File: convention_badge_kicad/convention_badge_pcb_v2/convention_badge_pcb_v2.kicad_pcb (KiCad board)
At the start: 4 copper layers, 90 x 98 mm, 56 parts, among them J1 USBC, J2 Conn_01x03_Pin, J3 3.7V Battery, J4 Conn_01x07_Pin, J5 Conn_01x07_Pin, Q1 AO3401A, SW1 SW4X2, SW2 SW4X2, SW3 SW_Push, SW4 SW_Push, SW5 SW_Push, SW6 SW4X2, U1 ESP32-C3-WROOM-02, U2 FS8205A, U3 TP4056, U4 DW01A, U5 TLV75733PDBV

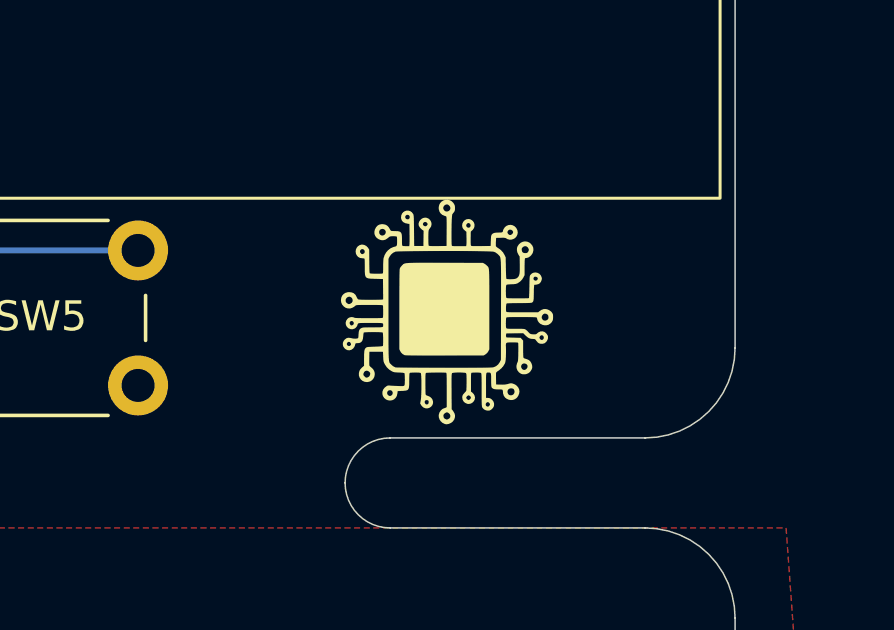
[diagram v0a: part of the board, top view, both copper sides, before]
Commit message: submitted to jlcpcb
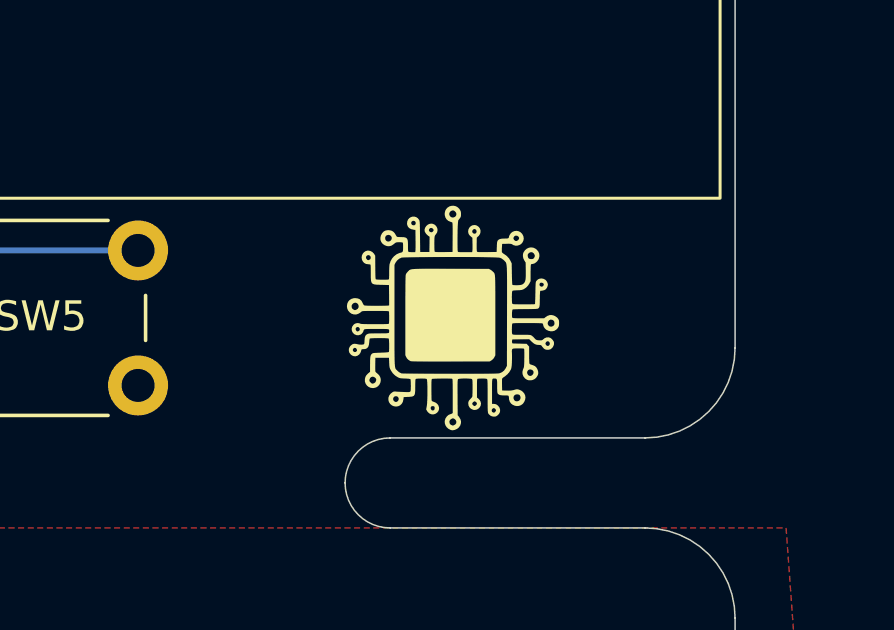
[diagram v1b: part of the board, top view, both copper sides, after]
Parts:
- moved G*** 0.28 mm to (190.2, 123.0)
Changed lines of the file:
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@@
 		(allow_soldermask_bridges_in_footprints no)
 		(tenting front back)
+		(aux_axis_origin 109.6 149)
+		(grid_origin 109.6 149)
 		(pcbplotparams
 			(layerselection 0x00000000_00000000_55555555_575555ff)
@@
 	(footprint "LOGO"
 		(layer "F.Cu")
-		(at 190 122.8)
+		(at 190.2 123)
 		(property "Reference" "G***"
 			(at 0 0 0)
@@
 			)
 		)
+		(property "LCSC" "C2337"
+			(at 0 0 0)
+			(unlocked yes)
+			(layer "F.Fab")
+			(hide yes)
+			(effects
+				(font
+					(size 1 1)
+					(thickness 0.15)
+				)
+			)
+		)
 		(property ki_fp_filters "Connector*:*_1x??_*")
 		(sheetname "/")
@@
 			)
 		)
+		(property "LCSC" ""
+			(at 0 0 0)
+			(unlocked yes)
+			(layer "F.Fab")
+			(hide yes)
+			(effects
+				(font
+					(size 1 1)
+					(thickness 0.15)
+				)
+			)
+		)
 		(property ki_fp_filters "Connector*:*_1x??_*")
 		(sheetname "/")
@@
 			)
 		)
+		(property "LCSC" ""
+			(at 0 0 270)
+			(unlocked yes)
+			(layer "F.Fab")
+			(hide yes)
+			(effects
+				(font
+					(size 1 1)
+					(thickness 0.15)
+				)
+			)
+		)
 		(property ki_fp_filters "Connector*:*_1x??_*")
 		(sheetname "/")
@@
 			)
 		)
-		(property "LCSC" " C318884"
+		(property "LCSC" "C318884"
 			(at 0 0 0)
 			(unlocked yes)
@@
 			)
 		)
-		(property "LCSC" "C1590"
+		(property "LCSC" "C14663"
 			(at 0 0 0)
 			(unlocked yes)
@@
 			)
 		)
-		(property "LCSC" " C485517"
+		(property "LCSC" "C485517"
 			(at 0 0 180)
 			(unlocked yes)
@@
 			)
 		)
-		(property "LCSC" "C1590"
+		(property "LCSC" "C14663"
 			(at 0 0 270)
 			(unlocked yes)
@@
 			)
 		)
-		(property "LCSC" "C2287"
+		(property "LCSC" "C2290"
 			(at 0 0 0)
 			(unlocked yes)
@@
 			)
 		)
-		(property "LCSC" " C351410"
+		(property "LCSC" "C351410"
 			(at 0 0 0)
 			(unlocked yes)
@@
 			)
 		)
-		(property "LCSC" " C318884"
+		(property "LCSC" "C318884"
 			(at 0 0 0)
 			(unlocked yes)
@@
 			)
 		)
-		(property "LCSC" "C1590"
+		(property "LCSC" "C14663"
 			(at 0 0 270)
 			(unlocked yes)
@@
 			)
 		)
-		(property "LCSC" "C1607"
+		(property "LCSC" "C23630"
 			(at 0 0 90)
 			(unlocked yes)
@@
 			)
 		)
-		(property "LCSC" "C1607"
+		(property "LCSC" "C23630"
 			(at 0 0 90)
 			(unlocked yes)
@@
 			)
 		)
-		(property "LCSC" "C1590"
+		(property "LCSC" "C14663"
 			(at 0 0 270)
 			(unlocked yes)
@@
 			)
 		)
-		(property "LCSC" " C318884"
+		(property "LCSC" "C318884"
 			(at 0 0 0)
 			(unlocked yes)
